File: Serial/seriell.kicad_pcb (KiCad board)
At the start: 2 copper layers, 136 x 62 mm, 31 parts, among them J1 Conn_01x10_Pin, J10 Conn_01x06, J11 Conn_01x06, J12 TTL, J13 Conn_01x10_Pin, J14 Conn_01x10_Pin, J15 Conn_01x10_Pin, J16 Conn_01x10_Pin, J17 Conn_01x10_Pin, J18 Conn_01x10_Pin, J2 Conn_01x10_Pin, J20 Auslesen, J3 Conn_01x10_Pin, J4 Conn_01x10_Pin, J5 Conn_01x10_Pin, J6 Conn_01x10_Pin, J7 Conn_02x04_Counter_Clockwise, J8 BT, U1 WeMos_D1_mini

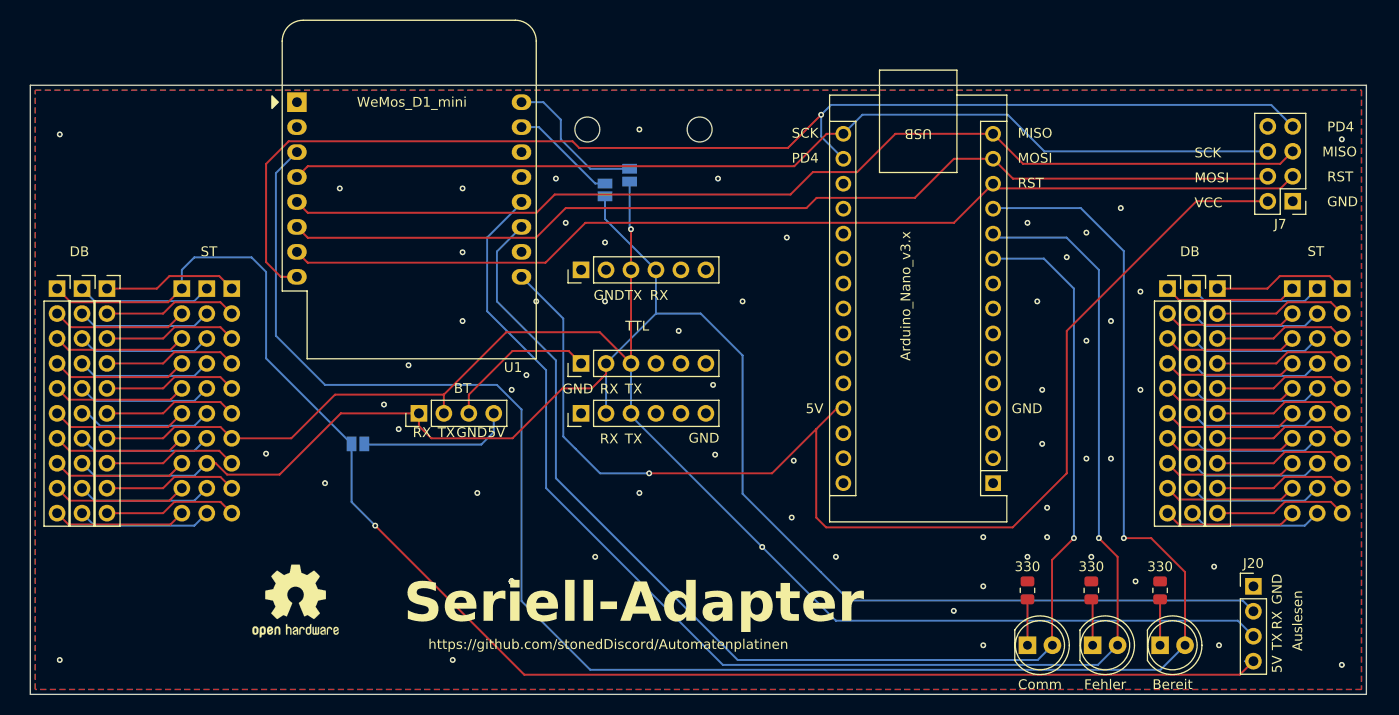
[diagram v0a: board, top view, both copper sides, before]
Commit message: esp
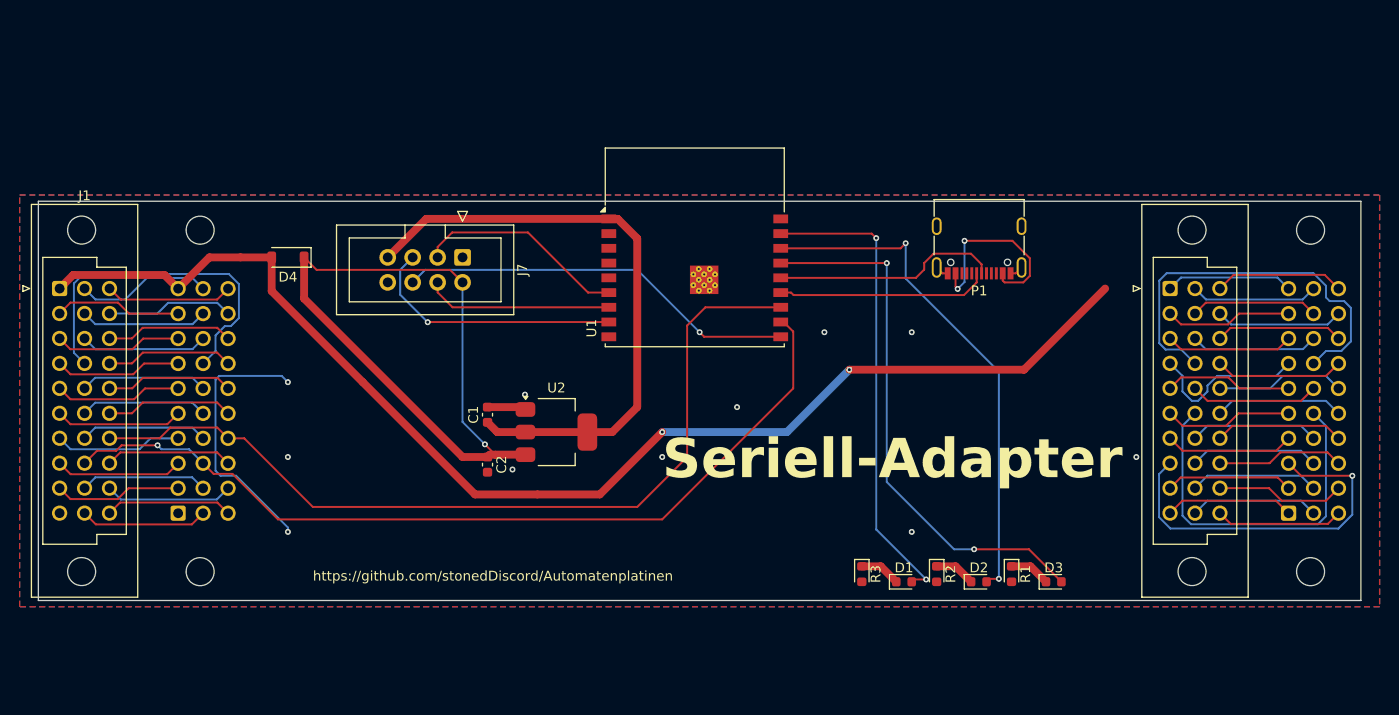
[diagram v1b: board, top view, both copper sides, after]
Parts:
- removed A1: Arduino_Nano_v3.x, Module:Arduino_Nano
- removed J10, J11: Conn_01x06, Connector_PinHeader_2.54mm:PinHeader_1x06_P2.54mm_Vertical
- removed J12: TTL, Connector_PinHeader_2.54mm:PinHeader_1x06_P2.54mm_Vertical
- removed J13, J14, J15, J16, J17, J18, J5, J6: Conn_01x10_Pin, Connector_PinSocket_2.54mm:PinSocket_1x10_P2.54mm_Vertical
- removed J20: Auslesen, Connector_PinHeader_2.54mm:PinHeader_1x04_P2.54mm_Vertical
- removed J8: BT, Connector_PinHeader_2.54mm:PinHeader_1x04_P2.54mm_Vertical
- removed JP1: Bluetooth, Jumper:SolderJumper-2_P1.3mm_Open_Pad1.0x1.5mm
- removed JP2: RX, Jumper:SolderJumper-2_P1.3mm_Open_Pad1.0x1.5mm
- removed JP3: TX, Jumper:SolderJumper-2_P1.3mm_Open_Pad1.0x1.5mm
- removed REF**: OSHW-Logo2_9.8x8mm_SilkScreen, Symbol:OSHW-Logo2_9.8x8mm_SilkScreen
- removed REF**: WEEE-Logo_8.4x12mm_SilkScreen, Symbol:WEEE-Logo_8.4x12mm_SilkScreen
- added C1: 10uF, Capacitor_SMD:C_0603_1608Metric, F.Cu at (129.5, 112.5)
- added C2: 10uF, Capacitor_SMD:C_0603_1608Metric, F.Cu at (129.5, 117.6)
- added D4: D, Diode_SMD:D_SOD-123, F.Cu at (109.2, 96.5)
- added P1: USB_C_Plug_USB2.0, Connector_USB:USB_C_Receptacle_G-Switch_GT-USB-7010ASV, F.Cu at (179.6, 94.4)
- added U2: AMS1117-3.3, Package_TO_SOT_SMD:SOT-223-3_TabPin2, F.Cu at (136.6, 114.3)
- D1, D2, D3: footprint LED_THT:LED_D5.0mm -> LED_SMD:LED_0603_1608Metric
- J1, J3: value Conn_01x10_Pin -> Datenbank; footprint Connector_PinSocket_2.54mm:PinSocket_1x10_P2.54mm_Vertical -> Connector_DIN:DIN41612_C3_3x10_Female_Vertical_THT
- J2, J4: value Conn_01x10_Pin -> Steuereinheit; footprint Connector_PinSocket_2.54mm:PinSocket_1x10_P2.54mm_Vertical -> Connector_DIN:DIN41612_R3_3x10_Male_Vertical_THT; moved to B.Cu
- J7: footprint Connector_PinHeader_2.54mm:PinHeader_2x04_P2.54mm_Vertical -> Connector_IDC:IDC-Header_2x04_P2.54mm_Vertical
- R1, R2, R3: footprint Resistor_SMD:R_0805_2012Metric -> LED_SMD:LED_0603_1608Metric
- U1: value WeMos_D1_mini -> ESP32-C3-WROOM-02; footprint Module:WEMOS_D1_mini_light -> RF_Module:ESP32-C3-WROOM-02
- moved J3 108.2 mm to (199.0, 99.7)
- moved J7 84.7 mm to (127.0, 96.5), turned to -90 degrees
- moved U1 44.3 mm to (150.6, 98.6)
- moved J4 26.0 mm to (211.1, 122.6)
- moved J2 24.9 mm to (98.0, 122.6)
- moved R3 16.9 mm to (167.6, 128.8), turned to -90 degrees
- moved R2 15.8 mm to (175.3, 128.8), turned to -90 degrees
- moved R1 15.2 mm to (182.9, 128.8), turned to -90 degrees
- moved D1 14.1 mm to (171.9, 129.5)
- moved D2 13.3 mm to (179.6, 129.5)
- moved D3 12.6 mm to (187.2, 129.5)
- moved J1 0.26 mm to (86.0, 99.7)
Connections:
- D1 pad 2: Net-(A1-D7) -> Net-(D1-A)
- D2 pad 2: Net-(A1-D8) -> Net-(D2-A)
- D3 pad 2: Net-(A1-D9) -> Net-(D3-A)
- U1 pad 1: unconnected-(U1-~{RST}-Pad1) -> +3.3V
- U1 pad 10: GND -> /SCK
- U1 pad 11: Net-(A1-D7) -> RX
- U1 pad 12: Net-(A1-D8) -> TX
- U1 pad 13: unconnected-(U1-SDA/D2-Pad13) -> Net-(P1-D-)
- U1 pad 14: unconnected-(U1-SCL/D1-Pad14) -> Net-(P1-D+)
- U1 pad 15: Net-(JP2-B) -> Net-(D3-A)
- U1 pad 16: Net-(JP3-B) -> Net-(D2-A)
- U1 pad 3: Net-(A1-D9) -> unconnected-(U1-IO4-Pad3)
- U1 pad 4: /SCK -> unconnected-(U1-IO5-Pad4)
- U1 pad 5: /MISO -> unconnected-(U1-IO6-Pad5)
- U1 pad 6: /MOSI -> /CS
- U1 pad 7: /CS -> /MOSI
- U1 pad 8: +3.3V -> /MISO
- U1 pad 9: +5VA -> GND
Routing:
- net Net-(A1-D9): track 198.1 -> 0.00 mm, vias 1 -> 0
- net Net-(A1-D8): track 150.8 -> 0.00 mm, vias 1 -> 0
- net Net-(A1-D7): track 134.7 -> 0.00 mm, vias 1 -> 0
- net /MOSI: track 103.5 -> 19.1 mm
- net /CS: track 105.9 -> 21.6 mm
- net RX: track 171.1 -> 89.0 mm, vias 0 -> 1
- net /MISO: track 106.9 -> 26.7 mm, vias 0 -> 1
- net TX: track 158.7 -> 88.4 mm, vias 2 -> 0
- net +3.3V: track 127.6 -> 61.7 mm, vias 1 -> 0
- net /SCK: track 103.0 -> 40.8 mm, vias 0 -> 1
- net +5VA: track 128.8 -> 69.6 mm
- net Net-(D3-A): track 0.00 -> 55.1 mm, vias 0 -> 2
- net Net-(D2-A): track 0.00 -> 52.4 mm, vias 0 -> 2
- net Net-(D1-A): track 0.00 -> 48.3 mm, vias 0 -> 2
- net GND: track 29.4 -> 76.6 mm, vias 61 -> 11
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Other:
- board size 136 x 62 mm -> 134.6 x 40.6 mm
- board text removed: "5V"
- board text removed: "DB"
- board text removed: "GND"
- board text removed: "MISO"
- board text removed: "MOSI"
- board text removed: "PD4"
- board text removed: "RST"
- board text removed: "RX"
- board text removed: "SCK"
- board text removed: "ST"
- board text removed: "TX"
- board text removed: "VCC"
- board text removed: "Wemos <->DB"
- board text removed: "offen=aus"
- board text removed: "zu=an"
